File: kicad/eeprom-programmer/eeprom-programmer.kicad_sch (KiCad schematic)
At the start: 19 parts, among them J1 Conn_01x03_Male, J2 Conn_01x05_Male, J3 Conn_01x02_Male, J4 Conn_01x01, J5 Conn_01x03_Male, U1 74HC595, U2 74HC595, U3 28C256

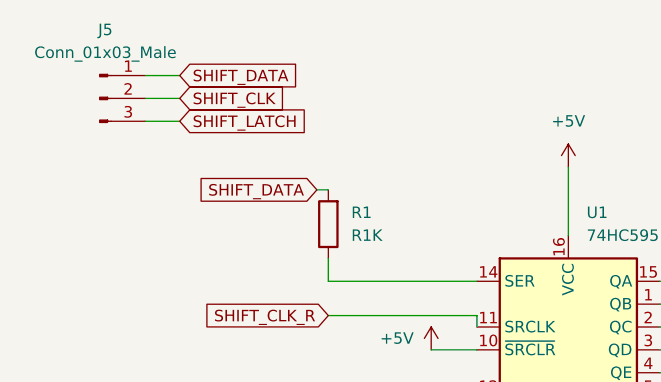
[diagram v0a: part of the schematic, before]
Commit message: PCB ready
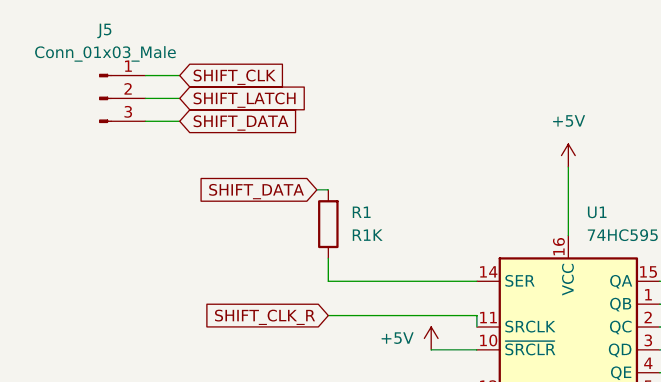
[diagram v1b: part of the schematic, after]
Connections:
- net SHIFT_CLK: now also J5.1 (Pin_1); no longer J5.2 (Pin_2)
- net SHIFT_DATA: now also J5.3 (Pin_3); no longer J5.1 (Pin_1)
- net SHIFT_LATCH: now also J5.2 (Pin_2); no longer J5.3 (Pin_3)
